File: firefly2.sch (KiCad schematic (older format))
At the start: 16 parts, among them P1 USB_B, P2 CONN_01X03, P3 CONN_01X04, P4 CONN_01X05, P5 CONN_01X01, U1 SAM_D11C, U2 RFM69CW, U3 MIC5504

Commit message: Footprint association
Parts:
- C1: footprint 0805-CAP -> SparkFun-Capacitors:0805
- C2, C3: footprint 0603-CAP -> SparkFun-Capacitors:0603
- D1, D2, D3, D4: footprint WS2812B -> SparkFun-LED:WS2812B
- P1: footprint (none) -> SparkFun-Connectors:USB-B-MICRO-SMD_V03
- P2: footprint (none) -> SparkFun-Connectors:1X03
- P3: footprint (none) -> SparkFun-Connectors:1X04
- P4: footprint (none) -> SparkFun-Connectors:1X05
- P5: footprint (none) -> SparkFun-Connectors:1X01
- R1: footprint (none) -> SparkFun-Resistors:0603
- U1: footprint (none) -> SMD_Packages:SOIC-14_N
- U2: footprint RFM69CW-XXXS2 -> SparkFun-RF:RFM69CW-XXXS2
- U3: footprint (none) -> TO_SOT_Packages_SMD:SOT-23-5
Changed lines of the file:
@@
 F 0 "U1" H 1400 1550 60  0000 C CNN
 F 1 "SAM_D11C" H 1450 1800 60  0000 C CNN
-F 2 "" H 1400 1550 60  0000 C CNN
+F 2 "SMD_Packages:SOIC-14_N" H 1400 1550 60  0001 C CNN
 F 3 "" H 1400 1550 60  0000 C CNN
 	1    1450 1800
@@
 F 0 "P1" H 1500 7150 50  0000 C CNN
 F 1 "USB_B" H 1250 7550 50  0000 C CNN
-F 2 "" V 1250 7250 50  0000 C CNN
+F 2 "SparkFun-Connectors:USB-B-MICRO-SMD_V03" V 1250 7250 50  0001 C CNN
 F 3 "" V 1250 7250 50  0000 C CNN
 	1    1300 7350
@@
 F 0 "P2" H 2100 7700 50  0000 C CNN
 F 1 "CONN_01X03" V 2200 7500 50  0000 C CNN
-F 2 "" H 2100 7500 50  0000 C CNN
+F 2 "SparkFun-Connectors:1X03" H 2100 7500 50  0001 C CNN
 F 3 "" H 2100 7500 50  0000 C CNN
 	1    2100 7500
@@
 Off board LED
 $Comp
-L +3V3 #PWR1
+L +3V3 #PWR01
 U 1 1 5A5421BD
 P 1000 1250
-F 0 "#PWR1" H 1000 1100 50  0001 C CNN
+F 0 "#PWR01" H 1000 1100 50  0001 C CNN
 F 1 "+3V3" H 1000 1390 50  0000 C CNN
 F 2 "" H 1000 1250 50  0000 C CNN
@@
 $EndComp
 $Comp
-L +5V #PWR5
+L +5V #PWR02
 U 1 1 5A54225C
 P 1900 7400
-F 0 "#PWR5" H 1900 7250 50  0001 C CNN
+F 0 "#PWR02" H 1900 7250 50  0001 C CNN
 F 1 "+5V" H 1900 7540 50  0000 C CNN
 F 2 "" H 1900 7400 50  0000 C CNN
@@
 $EndComp
 $Comp
-L GND #PWR6
+L GND #PWR03
 U 1 1 5A542285
 P 1900 7600
-F 0 "#PWR6" H 1900 7350 50  0001 C CNN
+F 0 "#PWR03" H 1900 7350 50  0001 C CNN
 F 1 "GND" H 1900 7450 50  0000 C CNN
 F 2 "" H 1900 7600 50  0000 C CNN
@@
 F 0 "P3" H 3000 7700 50  0000 C CNN
 F 1 "CONN_01X04" V 3100 7450 50  0000 C CNN
-F 2 "" H 3000 7450 50  0000 C CNN
+F 2 "SparkFun-Connectors:1X04" H 3000 7450 50  0001 C CNN
 F 3 "" H 3000 7450 50  0000 C CNN
 	1    3000 7450
@@
 ARM\nSerial Wire Debug
 $Comp
-L +3V3 #PWR7
+L +3V3 #PWR04
 U 1 1 5A54243D
 P 2800 7300
-F 0 "#PWR7" H 2800 7150 50  0001 C CNN
+F 0 "#PWR04" H 2800 7150 50  0001 C CNN
 F 1 "+3V3" H 2800 7440 50  0000 C CNN
 F 2 "" H 2800 7300 50  0000 C CNN
@@
 $EndComp
 $Comp
-L GND #PWR8
+L GND #PWR05
 U 1 1 5A542459
 P 2800 7600
-F 0 "#PWR8" H 2800 7350 50  0001 C CNN
+F 0 "#PWR05" H 2800 7350 50  0001 C CNN
 F 1 "GND" H 2800 7450 50  0000 C CNN
 F 2 "" H 2800 7600 50  0000 C CNN
@@
 	2800 7500 2500 7500
 $Comp
-L +5V #PWR3
+L +5V #PWR06
 U 1 1 5A5424FD
 P 1000 7150
-F 0 "#PWR3" H 1000 7000 50  0001 C CNN
+F 0 "#PWR06" H 1000 7000 50  0001 C CNN
 F 1 "+5V" H 1000 7290 50  0000 C CNN
 F 2 "" H 1000 7150 50  0000 C CNN
@@
 $EndComp
 $Comp
-L GND #PWR4
+L GND #PWR07
 U 1 1 5A542519
 P 1000 7450
-F 0 "#PWR4" H 1000 7200 50  0001 C CNN
+F 0 "#PWR07" H 1000 7200 50  0001 C CNN
 F 1 "GND" H 1000 7300 50  0000 C CNN
 F 2 "" H 1000 7450 50  0000 C CNN
@@
 	1000 7350 700  7350
 $Comp
-L GND #PWR11
+L GND #PWR08
 U 1 1 5A54267D
 P 3600 7500
-F 0 "#PWR11" H 3600 7250 50  0001 C CNN
+F 0 "#PWR08" H 3600 7250 50  0001 C CNN
 F 1 "GND" H 3600 7350 50  0000 C CNN
 F 2 "" H 3600 7500 50  0000 C CNN
@@
 $EndComp
 $Comp
-L +3V3 #PWR10
+L +3V3 #PWR09
 U 1 1 5A54269B
 P 3600 7200
-F 0 "#PWR10" H 3600 7050 50  0001 C CNN
+F 0 "#PWR09" H 3600 7050 50  0001 C CNN
 F 1 "+3V3" H 3600 7340 50  0000 C CNN
 F 2 "" H 3600 7200 50  0000 C CNN
@@
 $EndComp
 $Comp
-L +5V #PWR9
+L +5V #PWR010
 U 1 1 5A5426B9
 P 3600 7100
-F 0 "#PWR9" H 3600 6950 50  0001 C CNN
+F 0 "#PWR010" H 3600 6950 50  0001 C CNN
 F 1 "+5V" H 3600 7240 50  0000 C CNN
 F 2 "" H 3600 7100 50  0000 C CNN
@@
 Debug Power\nAccess
 $Comp
-L GND #PWR2
+L GND #PWR011
 U 1 1 5A542851
 P 1000 1350
-F 0 "#PWR2" H 1000 1100 50  0001 C CNN
+F 0 "#PWR011" H 1000 1100 50  0001 C CNN
 F 1 "GND" H 1000 1200 50  0000 C CNN
 F 2 "" H 1000 1350 50  0000 C CNN
@@
 F 0 "P4" H 3800 7600 50  0000 C CNN
 F 1 "CONN_01X05" V 3900 7300 50  0000 C CNN
-F 2 "" H 3800 7300 50  0000 C CNN
+F 2 "SparkFun-Connectors:1X05" H 3800 7300 50  0001 C CNN
 F 3 "" H 3800 7300 50  0000 C CNN
 	1    3800 7300
@@
 F 0 "U2" H 4500 2250 50  0000 L BNN
 F 1 "RFM69CW" H 4500 1075 50  0000 L BNN
-F 2 "RFM69CW-XXXS2" H 4930 1850 20  0001 C CNN
+F 2 "SparkFun-RF:RFM69CW-XXXS2" H 4930 1850 20  0001 C CNN
 F 3 "" H 4900 1700 60  0000 C CNN
 	1    4900 1700
@@
 $EndComp
 $Comp
-L GND #PWR13
+L GND #PWR012
 U 1 1 5A542675
 P 5500 1900
-F 0 "#PWR13" H 5500 1650 50  0001 C CNN
+F 0 "#PWR012" H 5500 1650 50  0001 C CNN
 F 1 "GND" H 5500 1750 50  0000 C CNN
 F 2 "" H 5500 1900 50  0000 C CNN
@@
 $EndComp
 $Comp
-L GND #PWR14
+L GND #PWR013
 U 1 1 5A542695
 P 5500 2100
-F 0 "#PWR14" H 5500 1850 50  0001 C CNN
+F 0 "#PWR013" H 5500 1850 50  0001 C CNN
 F 1 "GND" H 5500 1950 50  0000 C CNN
 F 2 "" H 5500 2100 50  0000 C CNN
@@
 F 0 "P5" H 4250 7550 50  0000 C CNN
 F 1 "CONN_01X01" V 4350 7450 50  0000 C CNN
-F 2 "" H 4250 7450 50  0000 C CNN
+F 2 "SparkFun-Connectors:1X01" H 4250 7450 50  0001 C CNN
 F 3 "" H 4250 7450 50  0000 C CNN
 	1    4250 7450
@@
 F 0 "D1" H 7260 1380 50  0000 L BNN
 F 1 "WS2812B" H 7250 750 50  0000 L BNN
-F 2 "WS2812B" H 7380 1200 20  0001 C CNN
+F 2 "SparkFun-LED:WS2812B" H 7380 1200 20  0001 C CNN
 F 3 "" H 7350 1050 60  0000 C CNN
 	1    7350 1050
@@
 F 0 "D2" H 7260 2180 50  0000 L BNN
 F 1 "WS2812B" H 7250 1550 50  0000 L BNN
-F 2 "WS2812B" H 7380 2000 20  0001 C CNN
+F 2 "SparkFun-LED:WS2812B" H 7380 2000 20  0001 C CNN
 F 3 "" H 7350 1850 60  0000 C CNN
 	1    7350 1850
@@
 F 0 "D3" H 7260 2980 50  0000 L BNN
 F 1 "WS2812B" H 7250 2350 50  0000 L BNN
-F 2 "WS2812B" H 7380 2800 20  0001 C CNN
+F 2 "SparkFun-LED:WS2812B" H 7380 2800 20  0001 C CNN
 F 3 "" H 7350 2650 60  0000 C CNN
 	1    7350 2650
@@
 F 0 "D4" H 7260 3780 50  0000 L BNN
 F 1 "WS2812B" H 7250 3150 50  0000 L BNN
-F 2 "WS2812B" H 7380 3600 20  0001 C CNN
+F 2 "SparkFun-LED:WS2812B" H 7380 3600 20  0001 C CNN
 F 3 "" H 7350 3450 60  0000 C CNN
 	1    7350 3450
@@
 $EndComp
 $Comp
-L +5V #PWR15
+L +5V #PWR014
 U 1 1 5A543862
 P 7150 850
-F 0 "#PWR15" H 7150 700 50  0001 C CNN
+F 0 "#PWR014" H 7150 700 50  0001 C CNN
 F 1 "+5V" H 7150 990 50  0000 C CNN
 F 2 "" H 7150 850 50  0000 C CNN
@@
 $EndComp
 $Comp
-L +5V #PWR16
+L +5V #PWR015
 U 1 1 5A54388C
 P 7150 1650
-F 0 "#PWR16" H 7150 1500 50  0001 C CNN
+F 0 "#PWR015" H 7150 1500 50  0001 C CNN
 F 1 "+5V" H 7150 1790 50  0000 C CNN
 F 2 "" H 7150 1650 50  0000 C CNN
@@
 $EndComp
 $Comp
-L +5V #PWR17
+L +5V #PWR016
 U 1 1 5A543915
 P 7150 2450
-F 0 "#PWR17" H 7150 2300 50  0001 C CNN
+F 0 "#PWR016" H 7150 2300 50  0001 C CNN
 F 1 "+5V" H 7150 2590 50  0000 C CNN
 F 2 "" H 7150 2450 50  0000 C CNN
@@
 $EndComp
 $Comp
-L +5V #PWR18
+L +5V #PWR017
 U 1 1 5A543955
 P 7150 3250
-F 0 "#PWR18" H 7150 3100 50  0001 C CNN
+F 0 "#PWR017" H 7150 3100 50  0001 C CNN
 F 1 "+5V" H 7150 3390 50  0000 C CNN
 F 2 "" H 7150 3250 50  0000 C CNN
@@
 $EndComp
 $Comp
-L GND #PWR19
+L GND #PWR018
 U 1 1 5A54397F
 P 8050 1150
-F 0 "#PWR19" H 8050 900 50  0001 C CNN
+F 0 "#PWR018" H 8050 900 50  0001 C CNN
 F 1 "GND" H 8050 1000 50  0000 C CNN
 F 2 "" H 8050 1150 50  0000 C CNN
@@
 $EndComp
 $Comp
-L GND #PWR20
+L GND #PWR019
 U 1 1 5A5439A9
 P 8050 1950
-F 0 "#PWR20" H 8050 1700 50  0001 C CNN
+F 0 "#PWR019" H 8050 1700 50  0001 C CNN
 F 1 "GND" H 8050 1800 50  0000 C CNN
 F 2 "" H 8050 1950 50  0000 C CNN
@@
 $EndComp
 $Comp
-L GND #PWR21
+L GND #PWR020
 U 1 1 5A5439D3
 P 8050 2750
-F 0 "#PWR21" H 8050 2500 50  0001 C CNN
+F 0 "#PWR020" H 8050 2500 50  0001 C CNN
 F 1 "GND" H 8050 2600 50  0000 C CNN
 F 2 "" H 8050 2750 50  0000 C CNN
@@
 $EndComp
 $Comp
-L GND #PWR22
+L GND #PWR021
 U 1 1 5A543A27
 P 8050 3550
-F 0 "#PWR22" H 8050 3300 50  0001 C CNN
+F 0 "#PWR021" H 8050 3300 50  0001 C CNN
 F 1 "GND" H 8050 3400 50  0000 C CNN
 F 2 "" H 8050 3550 50  0000 C CNN
@@
 F 0 "R1" V 8280 850 50  0000 C CNN
 F 1 "220" V 8200 850 50  0000 C CNN
-F 2 "" V 8130 850 50  0000 C CNN
+F 2 "SparkFun-Resistors:0603" V 8130 850 50  0001 C CNN
 F 3 "" H 8200 850 50  0000 C CNN
 	1    8200 850
@@
 F 0 "U3" H 10400 1450 60  0000 C CNN
 F 1 "MIC5504" H 10400 1000 60  0000 C CNN
-F 2 "" H 10400 1000 60  0000 C CNN
+F 2 "TO_SOT_Packages_SMD:SOT-23-5" H 10400 1000 60  0001 C CNN
 F 3 "" H 10400 1000 60  0000 C CNN
 	1    10400 1050
@@
 $EndComp
 $Comp
-L GND #PWR23
+L GND #PWR022
 U 1 1 5A5473E5
 P 9800 1150
-F 0 "#PWR23" H 9800 900 50  0001 C CNN
+F 0 "#PWR022" H 9800 900 50  0001 C CNN
 F 1 "GND" H 9800 1000 50  0000 C CNN
 F 2 "" H 9800 1150 50  0000 C CNN
@@
 $EndComp
 $Comp
-L +5V #PWR24
+L +5V #PWR023
 U 1 1 5A547413
 P 10000 750
-F 0 "#PWR24" H 10000 600 50  0001 C CNN
+F 0 "#PWR023" H 10000 600 50  0001 C CNN
 F 1 "+5V" H 10000 890 50  0000 C CNN
 F 2 "" H 10000 750 50  0000 C CNN
@@
 $EndComp
 $Comp
-L +3V3 #PWR25
+L +3V3 #PWR024
 U 1 1 5A547441
 P 10950 950
-F 0 "#PWR25" H 10950 800 50  0001 C CNN
+F 0 "#PWR024" H 10950 800 50  0001 C CNN
 F 1 "+3V3" H 10950 1090 50  0000 C CNN
 F 2 "" H 10950 950 50  0000 C CNN
@@
 F 0 "C2" H 9860 965 50  0000 L BNN
 F 1 "1uF" H 9860 765 50  0000 L BNN
-F 2 "0603-CAP" H 9830 1000 20  0001 C CNN
+F 2 "SparkFun-Capacitors:0603" H 9830 1000 20  0001 C CNN
 F 3 "" H 9800 850 60  0000 C CNN
 	1    9800 850
@@
 F 0 "C3" H 11010 1165 50  0000 L BNN
 F 1 "1uF" H 11010 965 50  0000 L BNN
-F 2 "0603-CAP" H 10980 1200 20  0001 C CNN
+F 2 "SparkFun-Capacitors:0603" H 10980 1200 20  0001 C CNN
 F 3 "" H 10950 1050 60  0000 C CNN
 	1    10950 1050
@@
 $EndComp
 $Comp
-L GND #PWR26
+L GND #PWR025
 U 1 1 5A547D81
 P 10950 1250
-F 0 "#PWR26" H 10950 1000 50  0001 C CNN
+F 0 "#PWR025" H 10950 1000 50  0001 C CNN
 F 1 "GND" H 10950 1100 50  0000 C CNN
 F 2 "" H 10950 1250 50  0000 C CNN
@@
 F 0 "C1" H 9610 965 50  0000 L BNN
 F 1 "10uF" H 9610 765 50  0000 L BNN
-F 2 "0805-CAP" H 9580 1000 20  0001 C CNN
+F 2 "SparkFun-Capacitors:0805" H 9580 1000 20  0001 C CNN
 F 3 "" H 9550 850 60  0000 C CNN
 	1    9550 850
@@
 NoConn ~ 1400 7650
 $Comp
-L +3V3 #PWR12
+L +3V3 #PWR026
 U 1 1 5A54A758
 P 4300 1300
-F 0 "#PWR12" H 4300 1150 50  0001 C CNN
+F 0 "#PWR026" H 4300 1150 50  0001 C CNN
 F 1 "+3V3" H 4300 1440 50  0000 C CNN
 F 2 "" H 4300 1300 50  0000 C CNN

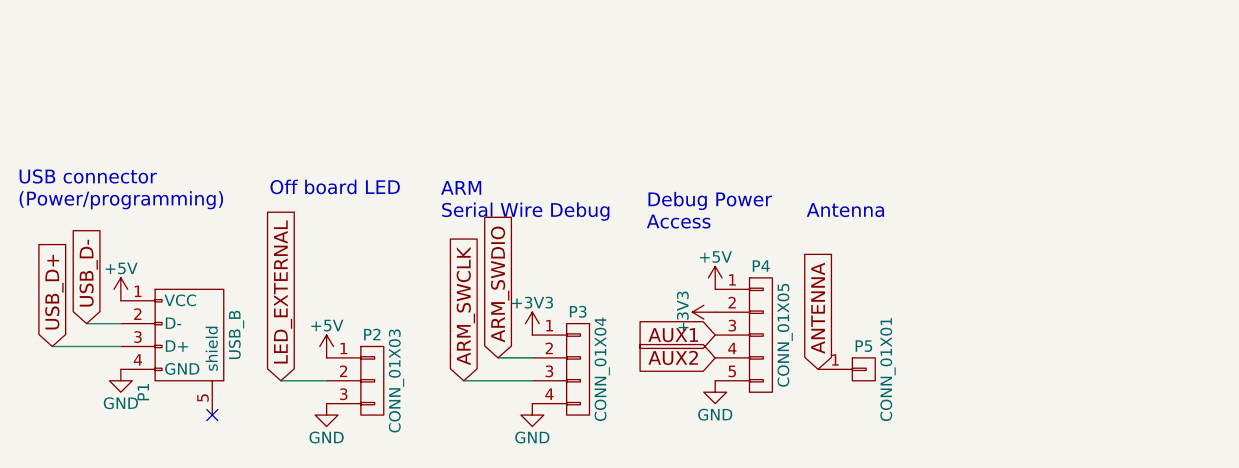
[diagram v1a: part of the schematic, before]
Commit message: First pass at placement
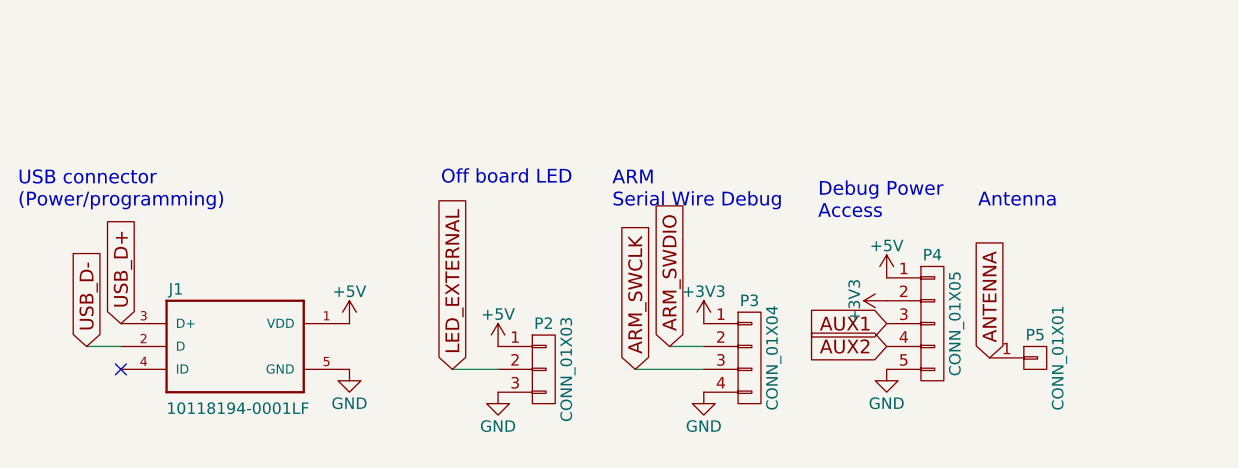
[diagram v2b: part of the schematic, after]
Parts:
- removed P1: USB_B, SparkFun-Connectors:USB-B-MICRO-SMD_V03, symbol USB_B_POWER_SUPPLY
- added J1: 10118194-0001LF, 10118194-0001LF:FRAMATOME_10118194-0001LF, symbol 10118194-0001LF
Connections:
- net +5V: now also J1.1 (VDD)
- net GND: now also J1.5 (GND)
- net USB_D+: now also J1.3 (D+)
- net USB_D-: now also J1.2 (D)
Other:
- moved on the sheet: P2, P3, P4, P5
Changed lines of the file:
@@
 LIBS:User-Submitted
 LIBS:adafruit
+LIBS:10118194-0001LF
 LIBS:firefly2-cache
 EELAYER 25 0
@@
 	1    0    0    -1
 $EndComp
-$Comp
-L USB_B_POWER_SUPPLY P1
-U 1 1 5A541EFE
-P 1300 7350
-F 0 "P1" H 1500 7150 50  0000 C CNN
-F 1 "USB_B" H 1250 7550 50  0000 C CNN
-F 2 "SparkFun-Connectors:USB-B-MICRO-SMD_V03" V 1250 7250 50  0001 C CNN
-F 3 "" V 1250 7250 50  0000 C CNN
-	1    1300 7350
-	0    1    1    0
-$EndComp
 Text Notes 7350 7500 0    60   ~ 0
 Firefly V2
@@
 L CONN_01X03 P2
 U 1 1 5A5420CD
-P 2100 7500
-F 0 "P2" H 2100 7700 50  0000 C CNN
-F 1 "CONN_01X03" V 2200 7500 50  0000 C CNN
-F 2 "SparkFun-Connectors:1X03" H 2100 7500 50  0001 C CNN
-F 3 "" H 2100 7500 50  0000 C CNN
-	1    2100 7500
+P 2850 7450
+F 0 "P2" H 2850 7650 50  0000 C CNN
+F 1 "CONN_01X03" V 2950 7450 50  0000 C CNN
+F 2 "SparkFun-Connectors:1X03" H 2850 7450 50  0001 C CNN
+F 3 "" H 2850 7450 50  0000 C CNN
+	1    2850 7450
 	1    0    0    -1
 $EndComp
 Text Notes 550  6750 0    60   ~ 0
 USB connector\n(Power/programming)
-Text Notes 1650 6700 0    60   ~ 0
+Text Notes 2400 6650 0    60   ~ 0
 Off board LED
 $Comp
@@
 L +5V #PWR02
 U 1 1 5A54225C
-P 1900 7400
-F 0 "#PWR02" H 1900 7250 50  0001 C CNN
-F 1 "+5V" H 1900 7540 50  0000 C CNN
-F 2 "" H 1900 7400 50  0000 C CNN
-F 3 "" H 1900 7400 50  0000 C CNN
-	1    1900 7400
+P 2650 7350
+F 0 "#PWR02" H 2650 7200 50  0001 C CNN
+F 1 "+5V" H 2650 7490 50  0000 C CNN
+F 2 "" H 2650 7350 50  0000 C CNN
+F 3 "" H 2650 7350 50  0000 C CNN
+	1    2650 7350
 	1    0    0    -1
 $EndComp
@@
 L GND #PWR03
 U 1 1 5A542285
-P 1900 7600
-F 0 "#PWR03" H 1900 7350 50  0001 C CNN
-F 1 "GND" H 1900 7450 50  0000 C CNN
-F 2 "" H 1900 7600 50  0000 C CNN
-F 3 "" H 1900 7600 50  0000 C CNN
-	1    1900 7600
-	1    0    0    -1
-$EndComp
-Text GLabel 1700 7500 1    60   Input ~ 0
+P 2650 7550
+F 0 "#PWR03" H 2650 7300 50  0001 C CNN
+F 1 "GND" H 2650 7400 50  0000 C CNN
+F 2 "" H 2650 7550 50  0000 C CNN
+F 3 "" H 2650 7550 50  0000 C CNN
+	1    2650 7550
+	1    0    0    -1
+$EndComp
+Text GLabel 2450 7450 1    60   Input ~ 0
 LED_EXTERNAL
 Wire Wire Line
-	1700 7500 1900 7500
+	2450 7450 2650 7450
 $Comp
 L CONN_01X04 P3
 U 1 1 5A5423D1
-P 3000 7450
-F 0 "P3" H 3000 7700 50  0000 C CNN
-F 1 "CONN_01X04" V 3100 7450 50  0000 C CNN
-F 2 "SparkFun-Connectors:1X04" H 3000 7450 50  0001 C CNN
-F 3 "" H 3000 7450 50  0000 C CNN
-	1    3000 7450
-	1    0    0    -1
-$EndComp
-Text Notes 2400 6800 0    60   ~ 0
+P 3750 7400
+F 0 "P3" H 3750 7650 50  0000 C CNN
+F 1 "CONN_01X04" V 3850 7400 50  0000 C CNN
+F 2 "SparkFun-Connectors:1X04" H 3750 7400 50  0001 C CNN
+F 3 "" H 3750 7400 50  0000 C CNN
+	1    3750 7400
+	1    0    0    -1
+$EndComp
+Text Notes 3150 6750 0    60   ~ 0
 ARM\nSerial Wire Debug
 $Comp
 L +3V3 #PWR04
 U 1 1 5A54243D
-P 2800 7300
-F 0 "#PWR04" H 2800 7150 50  0001 C CNN
-F 1 "+3V3" H 2800 7440 50  0000 C CNN
-F 2 "" H 2800 7300 50  0000 C CNN
-F 3 "" H 2800 7300 50  0000 C CNN
-	1    2800 7300
+P 3550 7250
+F 0 "#PWR04" H 3550 7100 50  0001 C CNN
+F 1 "+3V3" H 3550 7390 50  0000 C CNN
+F 2 "" H 3550 7250 50  0000 C CNN
+F 3 "" H 3550 7250 50  0000 C CNN
+	1    3550 7250
 	1    0    0    -1
 $EndComp
@@
 L GND #PWR05
 U 1 1 5A542459
-P 2800 7600
-F 0 "#PWR05" H 2800 7350 50  0001 C CNN
-F 1 "GND" H 2800 7450 50  0000 C CNN
-F 2 "" H 2800 7600 50  0000 C CNN
-F 3 "" H 2800 7600 50  0000 C CNN
-	1    2800 7600
-	1    0    0    -1
-$EndComp
-Text GLabel 2650 7400 1    60   Input ~ 0
+P 3550 7550
+F 0 "#PWR05" H 3550 7300 50  0001 C CNN
+F 1 "GND" H 3550 7400 50  0000 C CNN
+F 2 "" H 3550 7550 50  0000 C CNN
+F 3 "" H 3550 7550 50  0000 C CNN
+	1    3550 7550
+	1    0    0    -1
+$EndComp
+Text GLabel 3400 7350 1    60   Input ~ 0
 ARM_SWDIO
-Text GLabel 2500 7500 1    60   Input ~ 0
+Text GLabel 3250 7450 1    60   Input ~ 0
 ARM_SWCLK
 Wire Wire Line
-	2650 7400 2800 7400
-Wire Wire Line
-	2800 7500 2500 7500
+	3400 7350 3550 7350
+Wire Wire Line
+	3550 7450 3250 7450
 $Comp
 L +5V #PWR06
 U 1 1 5A5424FD
-P 1000 7150
-F 0 "#PWR06" H 1000 7000 50  0001 C CNN
-F 1 "+5V" H 1000 7290 50  0000 C CNN
-F 2 "" H 1000 7150 50  0000 C CNN
-F 3 "" H 1000 7150 50  0000 C CNN
-	1    1000 7150
+P 2000 7250
+F 0 "#PWR06" H 2000 7100 50  0001 C CNN
+F 1 "+5V" H 2000 7390 50  0000 C CNN
+F 2 "" H 2000 7250 50  0000 C CNN
+F 3 "" H 2000 7250 50  0000 C CNN
+	1    2000 7250
 	1    0    0    -1
 $EndComp
@@
 L GND #PWR07
 U 1 1 5A542519
-P 1000 7450
-F 0 "#PWR07" H 1000 7200 50  0001 C CNN
-F 1 "GND" H 1000 7300 50  0000 C CNN
-F 2 "" H 1000 7450 50  0000 C CNN
-F 3 "" H 1000 7450 50  0000 C CNN
-	1    1000 7450
-	1    0    0    -1
-$EndComp
-Text GLabel 850  7250 1    60   Input ~ 0
+P 2000 7450
+F 0 "#PWR07" H 2000 7200 50  0001 C CNN
+F 1 "GND" H 2000 7300 50  0000 C CNN
+F 2 "" H 2000 7450 50  0000 C CNN
+F 3 "" H 2000 7450 50  0000 C CNN
+	1    2000 7450
+	1    0    0    -1
+$EndComp
+Text GLabel 850  7350 1    60   Input ~ 0
 USB_D-
-Text GLabel 700  7350 1    60   Input ~ 0
+Text GLabel 1000 7250 1    60   Input ~ 0
 USB_D+
 Wire Wire Line
-	850  7250 1000 7250
-Wire Wire Line
-	1000 7350 700  7350
+	850  7350 1000 7350
 $Comp
 L GND #PWR08
 U 1 1 5A54267D
-P 3600 7500
-F 0 "#PWR08" H 3600 7250 50  0001 C CNN
-F 1 "GND" H 3600 7350 50  0000 C CNN
-F 2 "" H 3600 7500 50  0000 C CNN
-F 3 "" H 3600 7500 50  0000 C CNN
-	1    3600 7500
+P 4350 7450
+F 0 "#PWR08" H 4350 7200 50  0001 C CNN
+F 1 "GND" H 4350 7300 50  0000 C CNN
+F 2 "" H 4350 7450 50  0000 C CNN
+F 3 "" H 4350 7450 50  0000 C CNN
+	1    4350 7450
 	1    0    0    -1
 $EndComp
@@
 L +3V3 #PWR09
 U 1 1 5A54269B
-P 3600 7200
-F 0 "#PWR09" H 3600 7050 50  0001 C CNN
-F 1 "+3V3" H 3600 7340 50  0000 C CNN
-F 2 "" H 3600 7200 50  0000 C CNN
-F 3 "" H 3600 7200 50  0000 C CNN
-	1    3600 7200
+P 4350 7150
+F 0 "#PWR09" H 4350 7000 50  0001 C CNN
+F 1 "+3V3" H 4350 7290 50  0000 C CNN
+F 2 "" H 4350 7150 50  0000 C CNN
+F 3 "" H 4350 7150 50  0000 C CNN
+	1    4350 7150
 	0    -1   -1   0
 $EndComp
@@
 L +5V #PWR010
 U 1 1 5A5426B9
-P 3600 7100
-F 0 "#PWR010" H 3600 6950 50  0001 C CNN
-F 1 "+5V" H 3600 7240 50  0000 C CNN
-F 2 "" H 3600 7100 50  0000 C CNN
-F 3 "" H 3600 7100 50  0000 C CNN
-	1    3600 7100
-	1    0    0    -1
-$EndComp
-Text Notes 3300 6850 0    60   ~ 0
+P 4350 7050
+F 0 "#PWR010" H 4350 6900 50  0001 C CNN
+F 1 "+5V" H 4350 7190 50  0000 C CNN
+F 2 "" H 4350 7050 50  0000 C CNN
+F 3 "" H 4350 7050 50  0000 C CNN
+	1    4350 7050
+	1    0    0    -1
+$EndComp
+Text Notes 4050 6800 0    60   ~ 0
 Debug Power\nAccess
 $Comp
@@
 L CONN_01X05 P4
 U 1 1 5A54290F
-P 3800 7300
-F 0 "P4" H 3800 7600 50  0000 C CNN
-F 1 "CONN_01X05" V 3900 7300 50  0000 C CNN
-F 2 "SparkFun-Connectors:1X05" H 3800 7300 50  0001 C CNN
-F 3 "" H 3800 7300 50  0000 C CNN
-	1    3800 7300
-	1    0    0    -1
-$EndComp
-Text GLabel 3600 7300 0    60   Input ~ 0
+P 4550 7250
+F 0 "P4" H 4550 7550 50  0000 C CNN
+F 1 "CONN_01X05" V 4650 7250 50  0000 C CNN
+F 2 "SparkFun-Connectors:1X05" H 4550 7250 50  0001 C CNN
+F 3 "" H 4550 7250 50  0000 C CNN
+	1    4550 7250
+	1    0    0    -1
+$EndComp
+Text GLabel 4350 7250 0    60   Input ~ 0
 AUX1
-Text GLabel 3600 7400 0    60   Input ~ 0
+Text GLabel 4350 7350 0    60   Input ~ 0
 AUX2
 $Comp
@@
 L CONN_01X01 P5
 U 1 1 5A542715
-P 4250 7450
-F 0 "P5" H 4250 7550 50  0000 C CNN
-F 1 "CONN_01X01" V 4350 7450 50  0000 C CNN
-F 2 "SparkFun-Connectors:1X01" H 4250 7450 50  0001 C CNN
-F 3 "" H 4250 7450 50  0000 C CNN
-	1    4250 7450
-	1    0    0    -1
-$EndComp
-Text Notes 4000 6800 0    60   ~ 0
+P 5000 7400
+F 0 "P5" H 5000 7500 50  0000 C CNN
+F 1 "CONN_01X01" V 5100 7400 50  0000 C CNN
+F 2 "SparkFun-Connectors:1X01" H 5000 7400 50  0001 C CNN
+F 3 "" H 5000 7400 50  0000 C CNN
+	1    5000 7400
+	1    0    0    -1
+$EndComp
+Text Notes 4750 6750 0    60   ~ 0
 Antenna
-Text GLabel 4050 7450 1    60   Input ~ 0
+Text GLabel 4800 7400 1    60   Input ~ 0
 ANTENNA
 Text GLabel 5700 2000 2    60   Input ~ 0
@@
 Connection ~ 9800 750
 Connection ~ 9800 1050
-NoConn ~ 1400 7650
 $Comp
 L +3V3 #PWR026
@@
 	1    0    0    -1
 $EndComp
+$Comp
+L 10118194-0001LF J1
+U 1 1 5A59670D
+P 1500 7350
+F 0 "J1" H 1209 7571 50  0000 L BNN
+F 1 "10118194-0001LF" H 1199 7049 50  0000 L BNN
+F 2 "10118194-0001LF:FRAMATOME_10118194-0001LF" H 1500 7350 50  0001 L BNN
+F 3 "Amphenol" H 1500 7350 50  0001 L BNN
+F 4 "0.25 USD" H 1500 7350 50  0001 L BNN "Field4"
+F 5 "DIP-4 FCI" H 1500 7350 50  0001 L BNN "Field5"
+F 6 "Good" H 1500 7350 50  0001 L BNN "Field6"
+F 7 "10118194-0001LF" H 1500 7350 50  0001 L BNN "Field7"
+F 8 "CONN USB MICRO B RECPT SMT R/A" H 1500 7350 50  0001 L BNN "Field8"
+	1    1500 7350
+	1    0    0    -1
+$EndComp
+NoConn ~ 1000 7450
 $EndSCHEMATC
